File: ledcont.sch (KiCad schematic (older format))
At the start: 24 parts, among them J1 Screw_Terminal_01x02, J2 Screw_Terminal_01x02, U1 PAM2804, U2 MCP6002-xSN

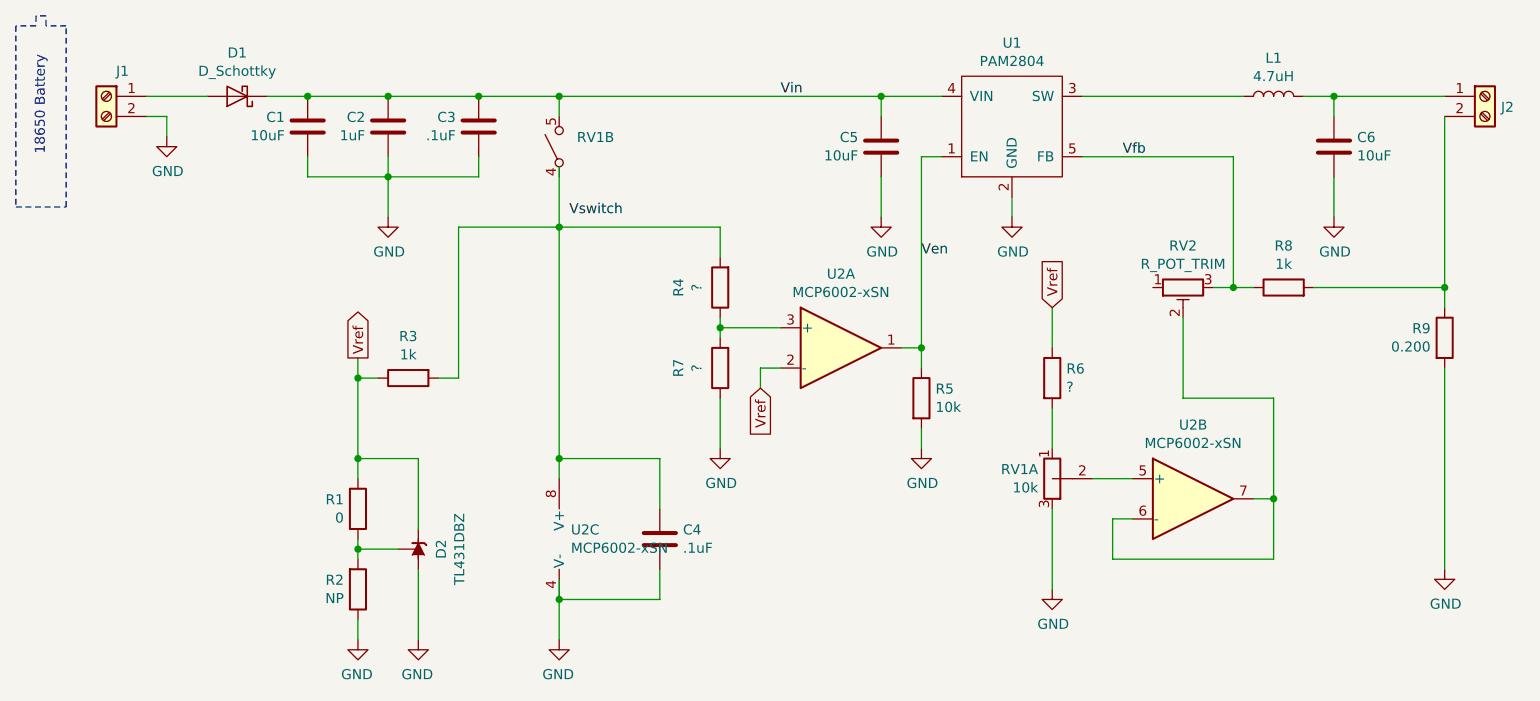
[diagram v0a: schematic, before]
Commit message: More board updates.
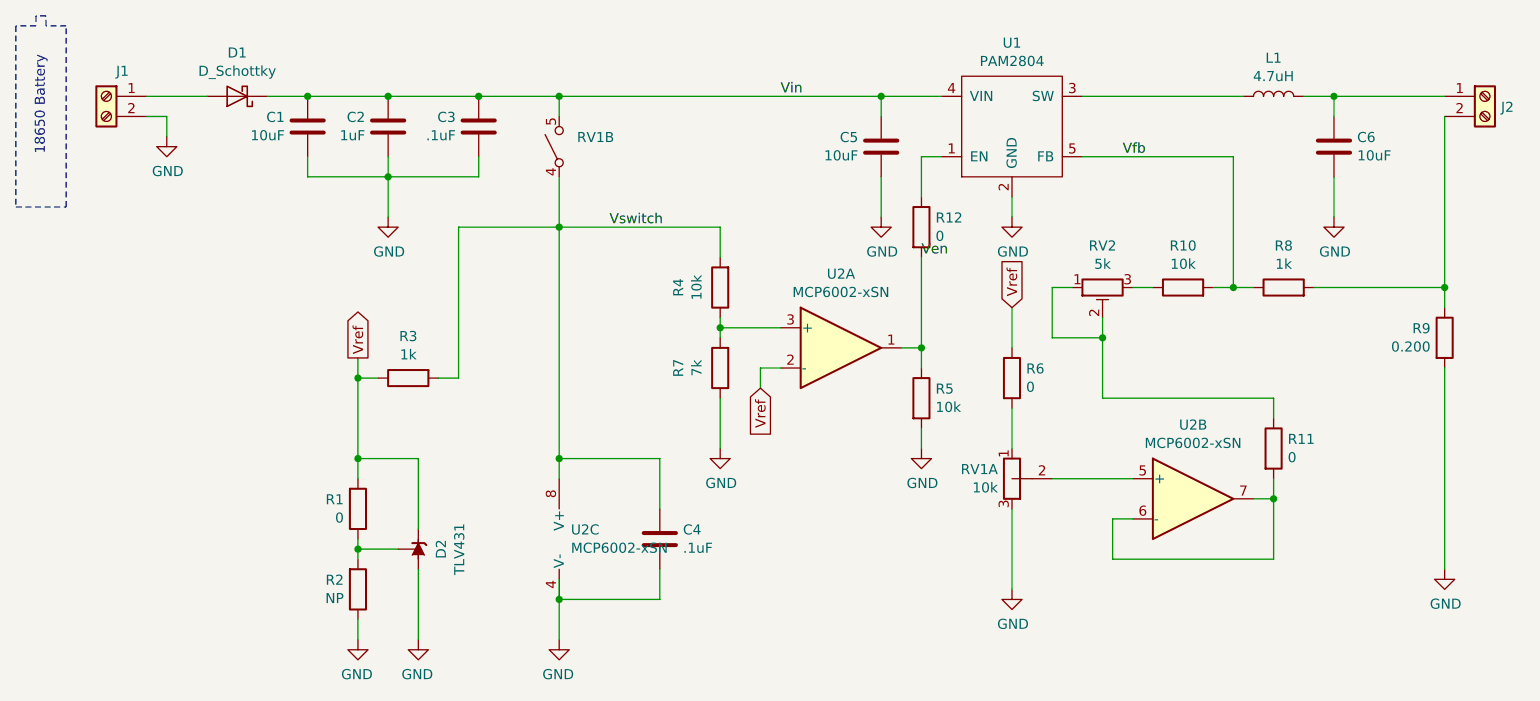
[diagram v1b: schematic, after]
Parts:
- added R10: 10k, Resistor_SMD:R_0603_1608Metric_Pad1.05x0.95mm_HandSolder, symbol Device:R
- added R11, R12: 0, Resistor_SMD:R_0603_1608Metric_Pad1.05x0.95mm_HandSolder, symbol Device:R
- D2: value TL431DBZ -> TLV431
- R1, R2, R3, R5: footprint Resistor_SMD:R_1206_3216Metric_Pad1.42x1.75mm_HandSolder -> Resistor_SMD:R_0603_1608Metric_Pad1.05x0.95mm_HandSolder
- R4: value ? -> 10k; footprint Resistor_SMD:R_1206_3216Metric_Pad1.42x1.75mm_HandSolder -> Resistor_SMD:R_0603_1608Metric_Pad1.05x0.95mm_HandSolder
- R6: value ? -> 0; footprint Resistor_SMD:R_1206_3216Metric_Pad1.42x1.75mm_HandSolder -> Resistor_SMD:R_0603_1608Metric_Pad1.05x0.95mm_HandSolder
- R7: value ? -> 7k; footprint Resistor_SMD:R_1206_3216Metric_Pad1.42x1.75mm_HandSolder -> Resistor_SMD:R_0603_1608Metric_Pad1.05x0.95mm_HandSolder
- RV2: value R_POT_TRIM -> 5k; footprint (none) -> ledcont:TC33X
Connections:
- net Ven: now also R12.2; no longer U1.1 (EN)
- net Vfb: now also R10.2; no longer RV2.3
- net Vswitch: now also C4.1, R3.2, R4.2, RV1.4, U2.8 (V+)
- net at U2.6 (-), U2.7: now also R11.2; no longer RV2.2
- net at RV2.1: now also RV2.2, R11.1
- new net: R12.1, U1.1 (EN)
- new net: R10.1, RV2.3
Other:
- moved on the sheet: R6, RV1A, RV2
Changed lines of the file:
@@
 L ledcont:R_POT_SPST RV1
 U 1 1 5C458CC6
-P 7450 4000
-F 0 "RV1" H 7380 3954 50  0000 R CNN
-F 1 "10k" H 7380 4045 50  0000 R CNN
-F 2 "ledcont:P091_S" H 7450 4000 50  0001 C CNN
-F 3 "~" H 7450 4000 50  0001 C CNN
-F 4 "P091S-FC20BR10K" H 700 -200 50  0001 C CNN "Part"
-	1    7450 4000
+P 7250 4000
+F 0 "RV1" H 7180 3954 50  0000 R CNN
+F 1 "10k" H 7180 4045 50  0000 R CNN
+F 2 "ledcont:P091_S" H 7250 4000 50  0001 C CNN
+F 3 "~" H 7250 4000 50  0001 C CNN
+F 4 "P091S-FC20BR10K" H 500 -200 50  0001 C CNN "Part"
+	1    7250 4000
 	1    0    0    1
 $EndComp
@@
 F 0 "R3" V 4043 3500 50  0000 C CNN
 F 1 "1k" V 4134 3500 50  0000 C CNN
-F 2 "Resistor_SMD:R_1206_3216Metric_Pad1.42x1.75mm_HandSolder" V 4180 3500 50  0001 C CNN
+F 2 "Resistor_SMD:R_0603_1608Metric_Pad1.05x0.95mm_HandSolder" V 4180 3500 50  0001 C CNN
 F 3 "~" H 4250 3500 50  0001 C CNN
 F 4 "1%" H -200 0   50  0001 C CNN "Tolerance"
@@
 F 0 "R1" H 3930 4104 50  0000 R CNN
 F 1 "0" H 3930 4195 50  0000 R CNN
-F 2 "Resistor_SMD:R_1206_3216Metric_Pad1.42x1.75mm_HandSolder" V 3930 4150 50  0001 C CNN
+F 2 "Resistor_SMD:R_0603_1608Metric_Pad1.05x0.95mm_HandSolder" V 3930 4150 50  0001 C CNN
 F 3 "~" H 4000 4150 50  0001 C CNN
 F 4 "1%" H 4000 4150 50  0001 C CNN "Tolerance"
@@
 F 0 "R2" H 3930 4504 50  0000 R CNN
 F 1 "NP" H 3930 4595 50  0000 R CNN
-F 2 "Resistor_SMD:R_1206_3216Metric_Pad1.42x1.75mm_HandSolder" V 3930 4550 50  0001 C CNN
+F 2 "Resistor_SMD:R_0603_1608Metric_Pad1.05x0.95mm_HandSolder" V 3930 4550 50  0001 C CNN
 F 3 "~" H 4000 4550 50  0001 C CNN
 F 4 "1%" H -200 0   50  0001 C CNN "Tolerance"
@@
 L Device:R R6
 U 1 1 5C482FDC
-P 7450 3500
-F 0 "R6" H 7520 3546 50  0000 L CNN
-F 1 "?" H 7520 3455 50  0000 L CNN
-F 2 "Resistor_SMD:R_1206_3216Metric_Pad1.42x1.75mm_HandSolder" V 7380 3500 50  0001 C CNN
-F 3 "~" H 7450 3500 50  0001 C CNN
-F 4 "RC1206FR-0720KL" H 700 -300 50  0001 C CNN "Part"
-	1    7450 3500
+P 7250 3500
+F 0 "R6" H 7320 3546 50  0000 L CNN
+F 1 "0" H 7320 3455 50  0000 L CNN
+F 2 "Resistor_SMD:R_0603_1608Metric_Pad1.05x0.95mm_HandSolder" V 7180 3500 50  0001 C CNN
+F 3 "~" H 7250 3500 50  0001 C CNN
+F 4 "RC1206FR-0720KL" H 500 -300 50  0001 C CNN "Part"
+	1    7250 3500
 	1    0    0    -1
 $EndComp
@@
 L power:GND #PWR011
 U 1 1 5C4859F5
-P 7450 4550
-F 0 "#PWR011" H 7450 4300 50  0001 C CNN
-F 1 "GND" H 7455 4377 50  0000 C CNN
-F 2 "" H 7450 4550 50  0001 C CNN
-F 3 "" H 7450 4550 50  0001 C CNN
-	1    7450 4550
-	1    0    0    -1
-$EndComp
-Text GLabel 7450 3150 1    50   Input ~ 0
+P 7250 4550
+F 0 "#PWR011" H 7250 4300 50  0001 C CNN
+F 1 "GND" H 7255 4377 50  0000 C CNN
+F 2 "" H 7250 4550 50  0001 C CNN
+F 3 "" H 7250 4550 50  0001 C CNN
+	1    7250 4550
+	1    0    0    -1
+$EndComp
+Text GLabel 7250 3150 1    50   Input ~ 0
 Vref
 Wire Wire Line
-	7450 3150 7450 3350
+	7250 3150 7250 3350
 Wire Notes Line
 	2300 1750 2300 2650
@@
 F 0 "R5" H 6870 3646 50  0000 L CNN
 F 1 "10k" H 6870 3555 50  0000 L CNN
-F 2 "Resistor_SMD:R_1206_3216Metric_Pad1.42x1.75mm_HandSolder" V 6730 3600 50  0001 C CNN
+F 2 "Resistor_SMD:R_0603_1608Metric_Pad1.05x0.95mm_HandSolder" V 6730 3600 50  0001 C CNN
 F 3 "~" H 6800 3600 50  0001 C CNN
 F 4 "1%" H 700 0   50  0001 C CNN "Tolerance"
@@
 Wire Wire Line
 	6800 3750 6800 3850
-Wire Wire Line
-	8350 3050 8250 3050
-Connection ~ 8350 3050
 Text GLabel 6000 3550 3    50   Input ~ 0
 Vref
@@
 	1    0    0    -1
 $EndComp
-Text Label 5050 2700 0    50   ~ 0
-Vswitch
 Text Label 6100 2100 0    50   ~ 0
 Vin
@@
 P 4300 4350
 F 0 "D2" H 4300 4236 50  0000 C CNN
-F 1 "TL431DBZ" H 4300 4145 50  0000 C CNN
+F 1 "TLV431" H 4300 4145 50  0000 C CNN
 F 2 "Package_TO_SOT_SMD:SOT-23" H 4300 4200 50  0001 C CIN
 F 3 "http://www.ti.com/lit/ds/symlink/tl431.pdf" H 4300 4350 50  0001 C CIN
@@
 	5000 2750 5000 3900
 Wire Wire Line
-	6800 2400 6800 3350
+	6800 2400 6800 2600
 Wire Wire Line
 	5000 2100 6600 2100
@@
 P 5800 3050
 F 0 "R4" V 6007 3050 50  0000 C CNN
-F 1 "?" V 5916 3050 50  0000 C CNN
-F 2 "Resistor_SMD:R_1206_3216Metric_Pad1.42x1.75mm_HandSolder" V 5730 3050 50  0001 C CNN
+F 1 "10k" V 5916 3050 50  0000 C CNN
+F 2 "Resistor_SMD:R_0603_1608Metric_Pad1.05x0.95mm_HandSolder" V 5730 3050 50  0001 C CNN
 F 3 "~" H 5800 3050 50  0001 C CNN
 F 4 "1%" H -2100 0   50  0001 C CNN "Tolerance"
@@
 P 5800 3450
 F 0 "R7" V 6007 3450 50  0000 C CNN
-F 1 "?" V 5916 3450 50  0000 C CNN
-F 2 "Resistor_SMD:R_1206_3216Metric_Pad1.42x1.75mm_HandSolder" V 5730 3450 50  0001 C CNN
+F 1 "7k" V 5916 3450 50  0000 C CNN
+F 2 "Resistor_SMD:R_0603_1608Metric_Pad1.05x0.95mm_HandSolder" V 5730 3450 50  0001 C CNN
 F 3 "~" H 5800 3450 50  0001 C CNN
 F 4 "RC1206FR-079K09L" H -1600 400 50  0001 C CNN "Part"
@@
 	7750 4200 7850 4200
 Wire Wire Line
-	7450 4150 7450 4550
-Wire Wire Line
-	7450 3650 7450 3850
-Wire Wire Line
-	7650 4000 7850 4000
+	7250 4150 7250 4550
+Wire Wire Line
+	7250 3650 7250 3850
+Wire Wire Line
+	7450 4000 7850 4000
 $Comp
 L Device:R_POT_TRIM RV2
 U 1 1 5C667481
+P 7700 3050
+F 0 "RV2" V 7493 3050 50  0000 C CNN
+F 1 "5k" V 7584 3050 50  0000 C CNN
+F 2 "ledcont:TC33X" H 7700 3050 50  0001 C CNN
+F 3 "~" H 7700 3050 50  0001 C CNN
+	1    7700 3050
+	0    -1   1    0
+$EndComp
+Wire Wire Line
+	7700 3200 7700 3300
+Wire Wire Line
+	7700 3600 8550 3600
+Wire Wire Line
+	8550 3600 8550 3700
+Connection ~ 8550 4100
+Wire Wire Line
+	5000 2500 5000 2750
+$Comp
+L Device:R R10
+U 1 1 5C5DEEB7
 P 8100 3050
-F 0 "RV2" V 7893 3050 50  0000 C CNN
-F 1 "R_POT_TRIM" V 7984 3050 50  0000 C CNN
-F 2 "" H 8100 3050 50  0001 C CNN
+F 0 "R10" V 8307 3050 50  0000 C CNN
+F 1 "10k" V 8216 3050 50  0000 C CNN
+F 2 "Resistor_SMD:R_0603_1608Metric_Pad1.05x0.95mm_HandSolder" V 8030 3050 50  0001 C CNN
 F 3 "~" H 8100 3050 50  0001 C CNN
+F 4 "1%" H 200 0   50  0001 C CNN "Tolerance"
+F 5 "RC1206FR-071KL" H 200 0   50  0001 C CNN "Part"
 	1    8100 3050
-	0    -1   1    0
-$EndComp
-Wire Wire Line
-	8100 3200 8100 3600
-Wire Wire Line
-	8100 3600 8550 3600
-Wire Wire Line
-	8550 3600 8550 4100
-Connection ~ 8550 4100
-Wire Wire Line
-	5000 2450 5000 2750
+	0    -1   -1   0
+$EndComp
+Wire Wire Line
+	8250 3050 8350 3050
+Connection ~ 8350 3050
+Wire Wire Line
+	7850 3050 7950 3050
+Wire Wire Line
+	7550 3050 7450 3050
+Wire Wire Line
+	7450 3050 7450 3300
+Wire Wire Line
+	7450 3300 7700 3300
+Connection ~ 7700 3300
+Wire Wire Line
+	7700 3300 7700 3600
+Text Label 5250 2750 0    50   ~ 0
+Vswitch
+$Comp
+L Device:R R11
+U 1 1 5C5FFECD
+P 8550 3850
+F 0 "R11" H 8620 3896 50  0000 L CNN
+F 1 "0" H 8620 3805 50  0000 L CNN
+F 2 "Resistor_SMD:R_0603_1608Metric_Pad1.05x0.95mm_HandSolder" V 8480 3850 50  0001 C CNN
+F 3 "~" H 8550 3850 50  0001 C CNN
+F 4 "RC1206FR-0720KL" H 1800 50  50  0001 C CNN "Part"
+	1    8550 3850
+	1    0    0    -1
+$EndComp
+Wire Wire Line
+	8550 4000 8550 4100
+$Comp
+L Device:R R12
+U 1 1 5C604BE5
+P 6800 2750
+F 0 "R12" H 6870 2796 50  0000 L CNN
+F 1 "0" H 6870 2705 50  0000 L CNN
+F 2 "Resistor_SMD:R_0603_1608Metric_Pad1.05x0.95mm_HandSolder" V 6730 2750 50  0001 C CNN
+F 3 "~" H 6800 2750 50  0001 C CNN
+F 4 "RC1206FR-0720KL" H 50  -1050 50  0001 C CNN "Part"
+	1    6800 2750
+	1    0    0    -1
+$EndComp
+Wire Wire Line
+	6800 2900 6800 3350
 $EndSCHEMATC
